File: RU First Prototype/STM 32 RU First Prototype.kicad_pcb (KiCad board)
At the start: 4 copper layers, 44.5 x 76.5 mm, 98 parts, among them J1 Conn_01x02, J10 Conn_01x02_Pin, J11 Conn_01x02_Pin, J12 1776113-2, J2 USB_C_Receptacle, J3 Conn_01x02_Pin, J4 Conn_01x04, J5 Conn_01x02_Pin, J7 1776113-2, J9 Conn_01x02_Pin, Q1 SISA96DN-T1, Q3 SISA96DN-T1, SW1 SW_SPDT, U1 STM32F412RGTx, U2 AMS1117-3.3, U3 MS5611, U4 KX134-1211, U5 W25Q16JVSS, U6 TCAN330, U7 TCAN330, Y1 Crystal_8Mhz

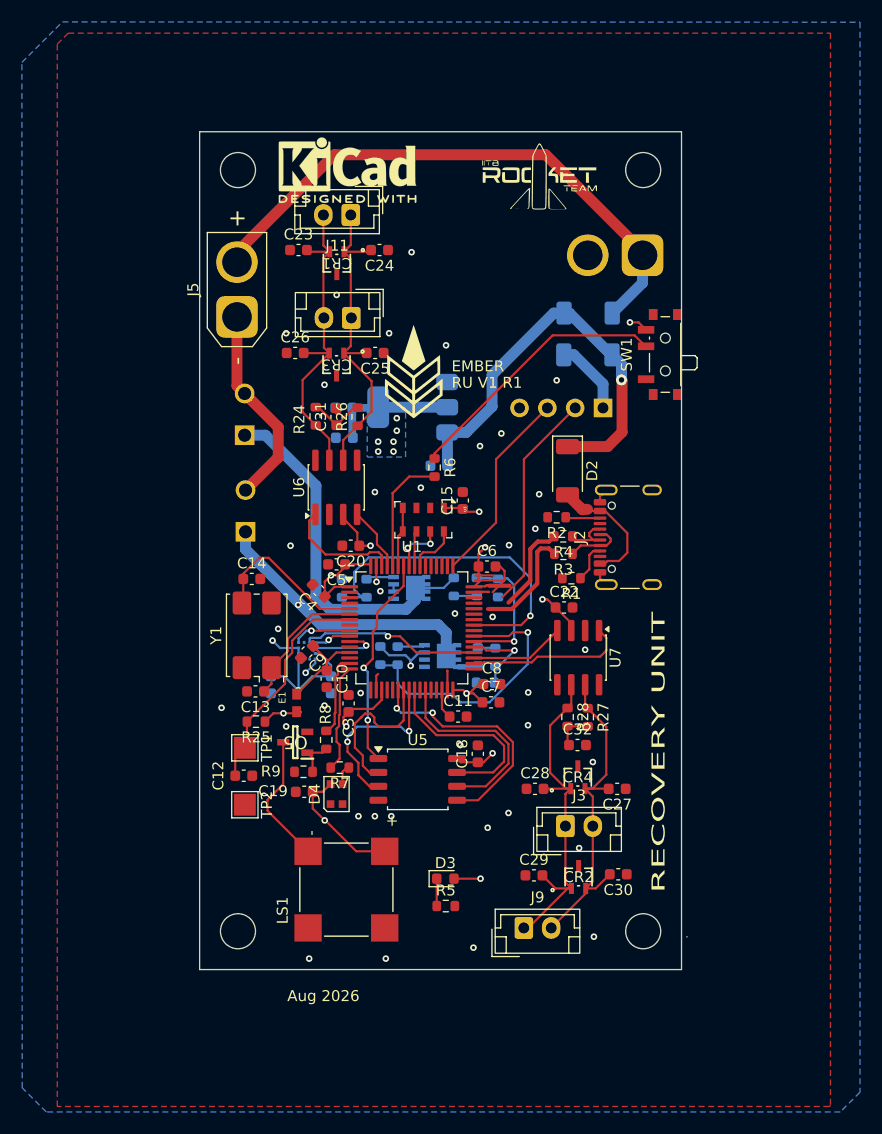
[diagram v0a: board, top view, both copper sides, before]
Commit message: Final touch done from my side
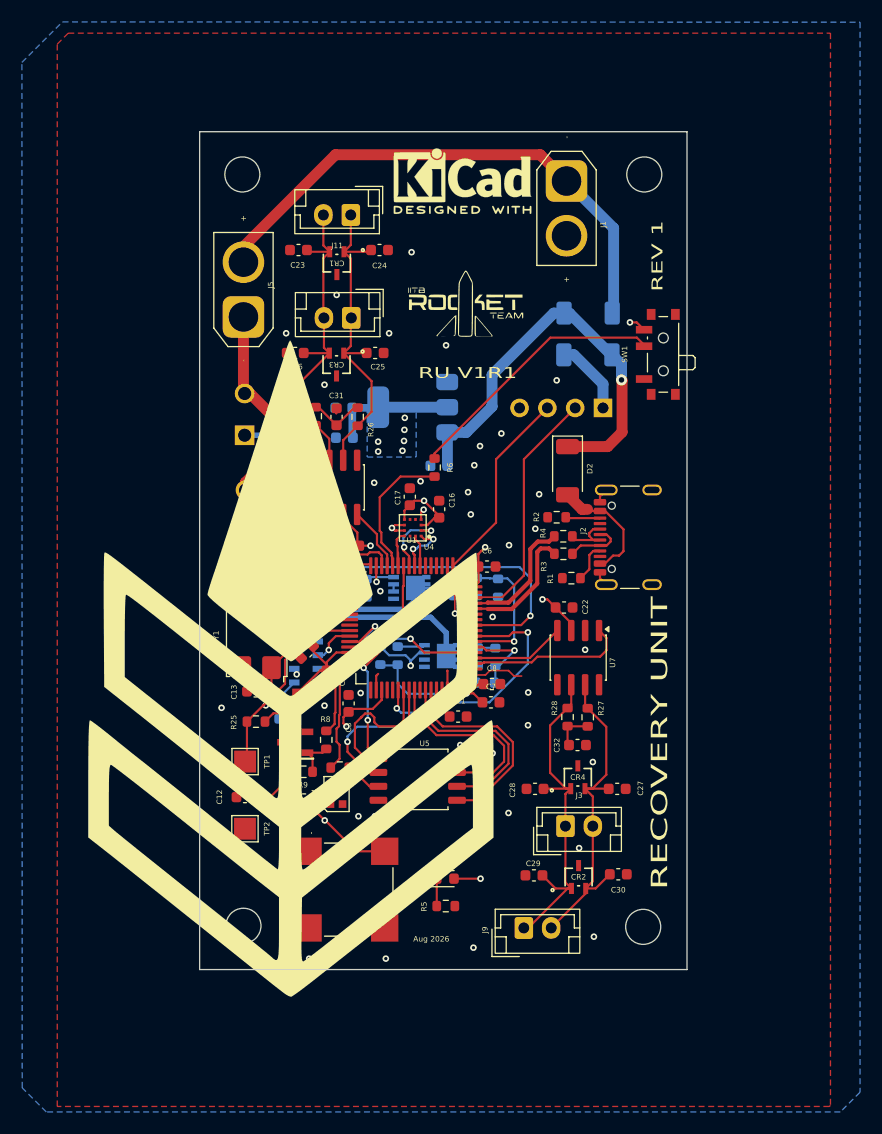
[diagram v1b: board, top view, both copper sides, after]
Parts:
- removed the G*** at (121.5, 76.5)
- added G***: LOGO, RT_Graphics:project_logo_huge.kicad_sym, F.Cu at (110.0, 104.2)
- C15, U3: moved to B.Cu
- C16, C17, J1, U4: moved to F.Cu
- moved C15 25.4 mm to (109.3, 107.3), turned to -90 degrees
- moved C17 21.4 mm to (121.2, 87.8), turned to 90 degrees
- moved C16 18.8 mm to (123.9, 89.0), turned to 90 degrees
- moved U3 16.8 mm to (111.7, 102.9), turned to 0 degrees
- moved U4 14.8 mm to (121.5, 90.7)
- moved G*** 13.4 mm to (126.3, 70.6)
- moved REF** 10.5 mm to (126.0, 59.0)
- moved J1 9.70 mm to (135.5, 59.0), turned to -90 degrees
- moved TP2 2.19 mm to (106.1, 118.1)
- moved C12 1.95 mm to (106.1, 115.2)
- moved TP1 1.26 mm to (106.2, 112.0)
- moved REF** 0.71 mm to (106.0, 127.0)
- moved C19 0.70 mm to (111.5, 115.5)
- moved J5 0.59 mm to (106.0, 71.4)
- moved REF** 0.57 mm to (105.9, 58.4)
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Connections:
- U1 pad 10: /KX_SDO -> /ALT_SDO
- U1 pad 11: /KX_SDI -> /ALT_SDI
- U1 pad 36: /KX_SCK -> /ALT_SCLK
- U1 pad 55: /ALT_SCLK -> /KX_SCK
- U1 pad 56: /ALT_SDO -> /KX_SDO
- U1 pad 57: /ALT_SDI -> /KX_SDI
- U1 pad 59: /ALT_CS -> /KX_CS
- U1 pad 9: /KX_CS -> /ALT_CS
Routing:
- net /KX_SCK: track 16.3 -> 2.89 mm, vias 1 -> 0
- net /ALT_SCLK: track 4.66 -> 16.7 mm, vias 0 -> 1
- net +3V3: track 83.7 -> 77.3 mm
- net /ALT_SDI: track 5.04 -> 10.7 mm, vias 2 -> 1
- net GND: track 25.4 -> 29.5 mm, vias 44 -> 48
- net /V_2S: track 53.1 -> 49.5 mm
- net /ALT_CS: track 5.45 -> 7.21 mm, vias 0 -> 1
- net /KX_SDO: track 3.45 -> 5.20 mm, vias 1 -> 2
- net /BOOT0: track 11.1 -> 12.5 mm
- net /D-: track 10.3 -> 11.5 mm
- net /NRST: track 21.4 -> 22.4 mm
- net /KX_CS: track 5.33 -> 4.45 mm, vias 1 -> 0
- net /ALT_SDO: track 3.20 -> 3.99 mm, vias 0 -> 1
- net /Main: track 31.7 -> 31.0 mm
- net /V_USB: track 12.0 -> 11.5 mm
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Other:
- outline, holes or cut-outs redrawn
- board text added: "Every av component has to have a cursed looking prototype - The person who has this r*t**ded idead called TSMBAS"
- board text added: "REV 1"
- board text added: "RU V1R1"
- board text removed: "EMBER"
- board text removed: "RU V1 R1"
